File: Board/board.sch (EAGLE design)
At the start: 37 parts, among them IC1 MCP2300X/SO, IC2 LM1117, U2 MAX11607EUA+T

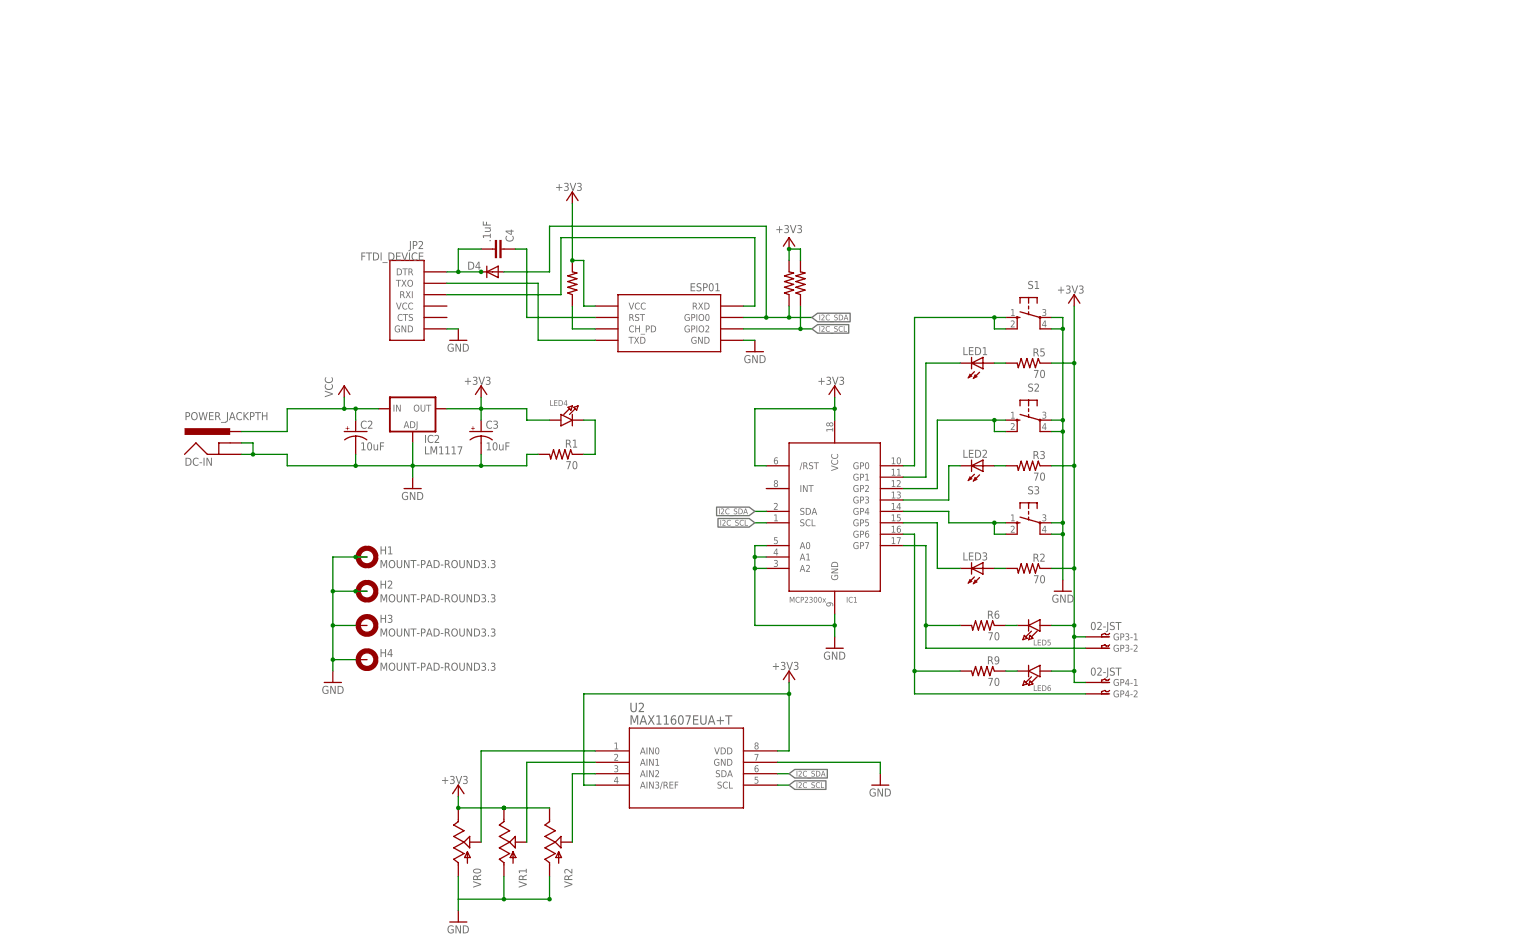
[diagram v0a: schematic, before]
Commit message: Finish routing PCB
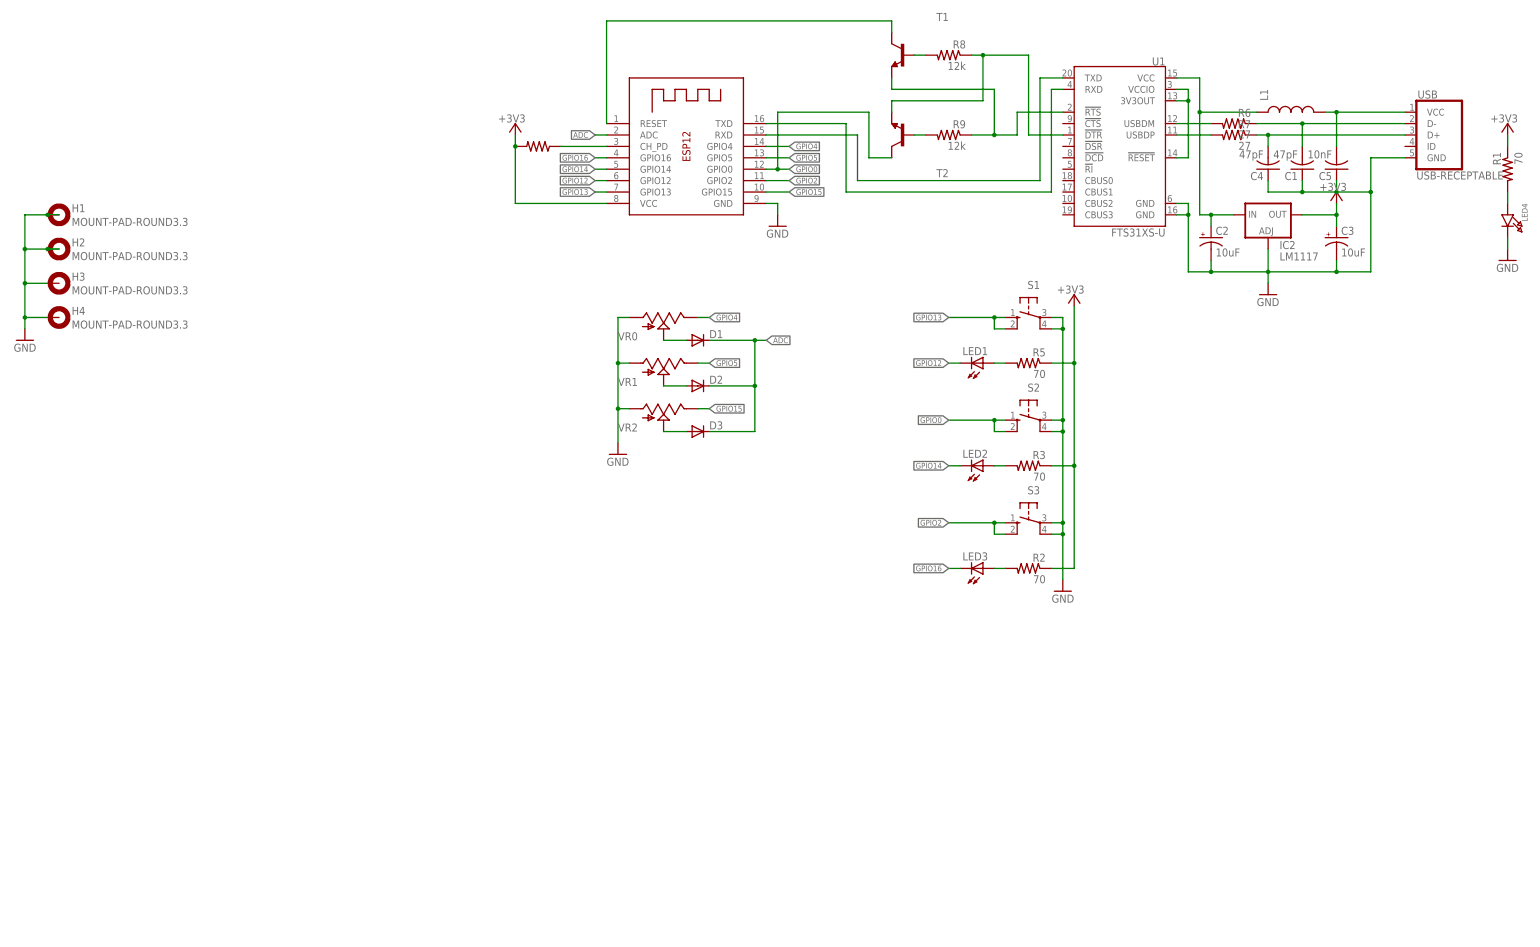
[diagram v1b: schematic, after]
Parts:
- removed D4: (no value), diode:DIODE-DO214AC
- removed DC-IN: POWER_JACKPTH, SparkFun-Connectors:POWER_JACKPTH
- removed ESP-01: ESP01, esp8266modules-pk:ESP01
- removed GP3, GP4: 02-JST, con-jst-xh:02-JST
- removed IC1: MCP2300X/SO, adafruit:MCP2300X/SO
- removed JP2: FTDI_DEVICE, SparkFun-Connectors:FTDI_DEVICE
- removed LED5, LED6: (no value), microbuilder:LED0805
- removed U2: MAX11607EUA+T, MAX11607:MAX11607EUA+T
- added C1: 47pF, rcl:C-USC0603
- added C5: 10nF, rcl:C-USC0603
- added D1, D2, D3: (no value), diode:DIODE-DO214AC
- added L1: (no value), SparkFun-Passives:INDUCTOR0805
- added T1, T2: (no value), transistor:MMBT918LT1-NPN-SOT23-BEC
- added U1: FTS31XS-U, SparkFun-DigitalIC:FT231XS
- added USB: USB-RECEPTABLE, daspilker:USB-RECEPTABLE
- added X1: (no value), adafruit:ESP-12
- C4: value .1uF -> 47pF; device SparkFun-Passives:CAP0603-CAP -> rcl:C-USC0603
- R6: value 70 -> 27
- R7: value 10k -> 27
- R8: value 10k -> 12k
- R9: value 70 -> 12k
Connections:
- removed net GP0: IC1.GP0, S1.S, S1.S1
- removed net GP1: IC1.GP1, LED1.C
- removed net GP2: IC1.GP2, S2.S, S2.S1
- removed net GP3: IC1.GP3, LED2.C
- removed net GP4: IC1.GP4, S3.S, S3.S1
- removed net GP5: IC1.GP5, LED3.C
- removed net GP6: GP3-2.1, IC1.GP7, R6.2
- removed net GP7: GP4-2.1, IC1.GP6, R9.2
- removed net I2C_SCL: ESP-01.GPIO2, IC1.SCL, R8.1, U2.SCL
- removed net I2C_SDA: D4.A, ESP-01.GPIO0, IC1.SDA, R7.1, U2.SDA
- removed net VCC: C2.+, DC-IN.PWR, IC2.IN
- new net ADC: D1.C, D2.C, D3.C, X1.ADC
- new net GPIO0: S2.S, S2.S1, T2.C, X1.GPIO0
- new net GPIO12: LED1.C, X1.GPIO12
- new net GPIO13: S1.S, S1.S1, X1.GPIO13
- new net GPIO14: LED2.C, X1.GPIO14
- new net GPIO15: VR2.E, X1.GPIO15
- new net GPIO16: LED3.C, X1.GPIO16
- new net GPIO2: S3.S, S3.S1, X1.GPIO2
- new net GPIO4: VR0.E, X1.GPIO4
- new net GPIO5: VR1.E, X1.GPIO5
- new net N$12: D3.A, VR2.S
- new net N$13: C1.2, R6.1, USB.D-
- new net N$14: R8.1, T2.E, U1.!DTR
- new net N$15: R9.1, T1.E, U1.!RTS
- new net N$16: R8.2, T1.B
- new net N$17: R9.2, T2.B
- new net N$19: U1.!RESET, U1.3V3OUT, U1.VCCIO
- new net N$20: C2.+, IC2.IN, L1.1, U1.VCC
- net +3V3: now also R1.1, X1.VCC; no longer ESP-01.VCC, GP3-1.1, GP4-1.1, IC1./RST, IC1.VCC, LED4.A, LED5.A, LED6.A, R7.2, R8.2, U2.AIN3/REF, U2.VDD, VR0.E, VR1.E, VR2.E
- net GND: now also C1.1, C4.1, C5.1, LED4.C, U1.GND@16, U1.GND@6, USB.GND, X1.GND; no longer DC-IN.GND, DC-IN.GNDBREAK, ESP-01.GND, IC1.A0, IC1.A1, IC1.A2, IC1.GND, JP2.GND, R1.2, U2.GND
- net N$1: now also X1.CH_PD; no longer ESP-01.CH_PD
- net N$11: now also D2.A, VR1.S; no longer LED6.C, R9.1
- net N$2: now also R7.1, USB.D+; no longer D4.C, JP2.DTR
- net N$3: now also R7.2, U1.USBDP; no longer U2.AIN2, VR2.S
- net N$4: now also LED4.A, R1.2; no longer U2.AIN1, VR1.S
- net N$5: now also D1.A; no longer U2.AIN0
- net N$7: now also C5.2, L1.2, USB.VCC; no longer LED4.C, R1.1
- net N$9: now also R6.2, U1.USBDM; no longer LED5.C, R6.1
- net RST: now also T1.C, X1.RESET; no longer C4.1, ESP-01.RST
- net RXI: now also U1.TXD, X1.RXD; no longer ESP-01.RXD, JP2.RXI
- net TXO: now also U1.RXD, X1.TXD; no longer ESP-01.TXD, JP2.TXO
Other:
- moved on the sheet: C2, C3, C4, H1, H2, H3, H4, IC2, LED4, R1, R6, R9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
